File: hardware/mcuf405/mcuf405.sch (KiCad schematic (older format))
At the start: 35 parts, among them J4 STM32WORLD_BASE, U1 STM32F405RGTx, U2 XC6206P332MR, Y1 16 MHz

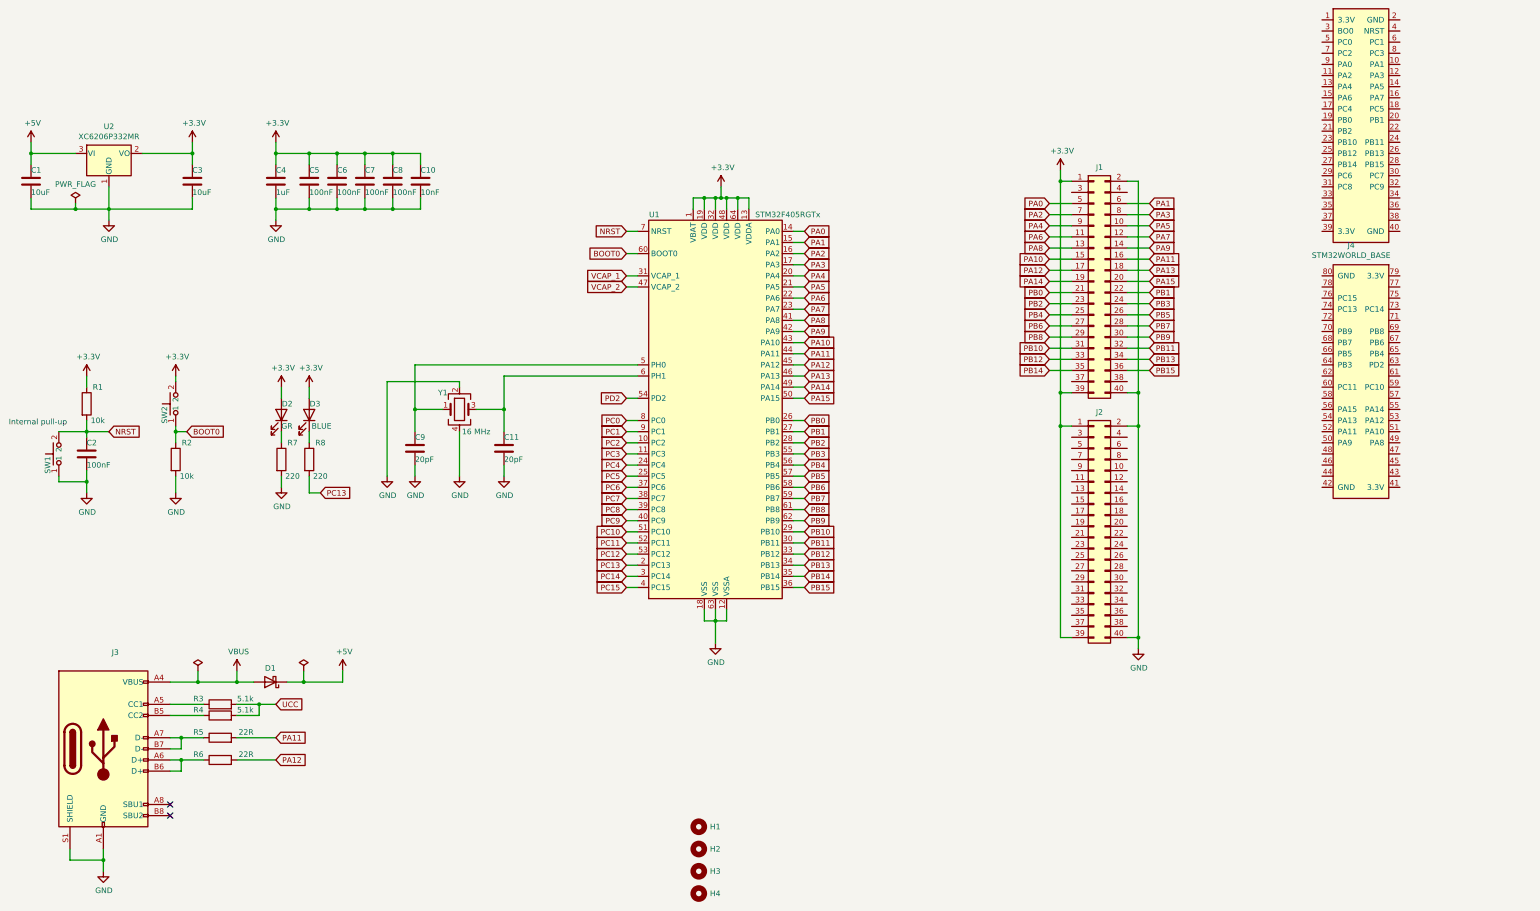
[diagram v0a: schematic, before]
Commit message: Hmmmm
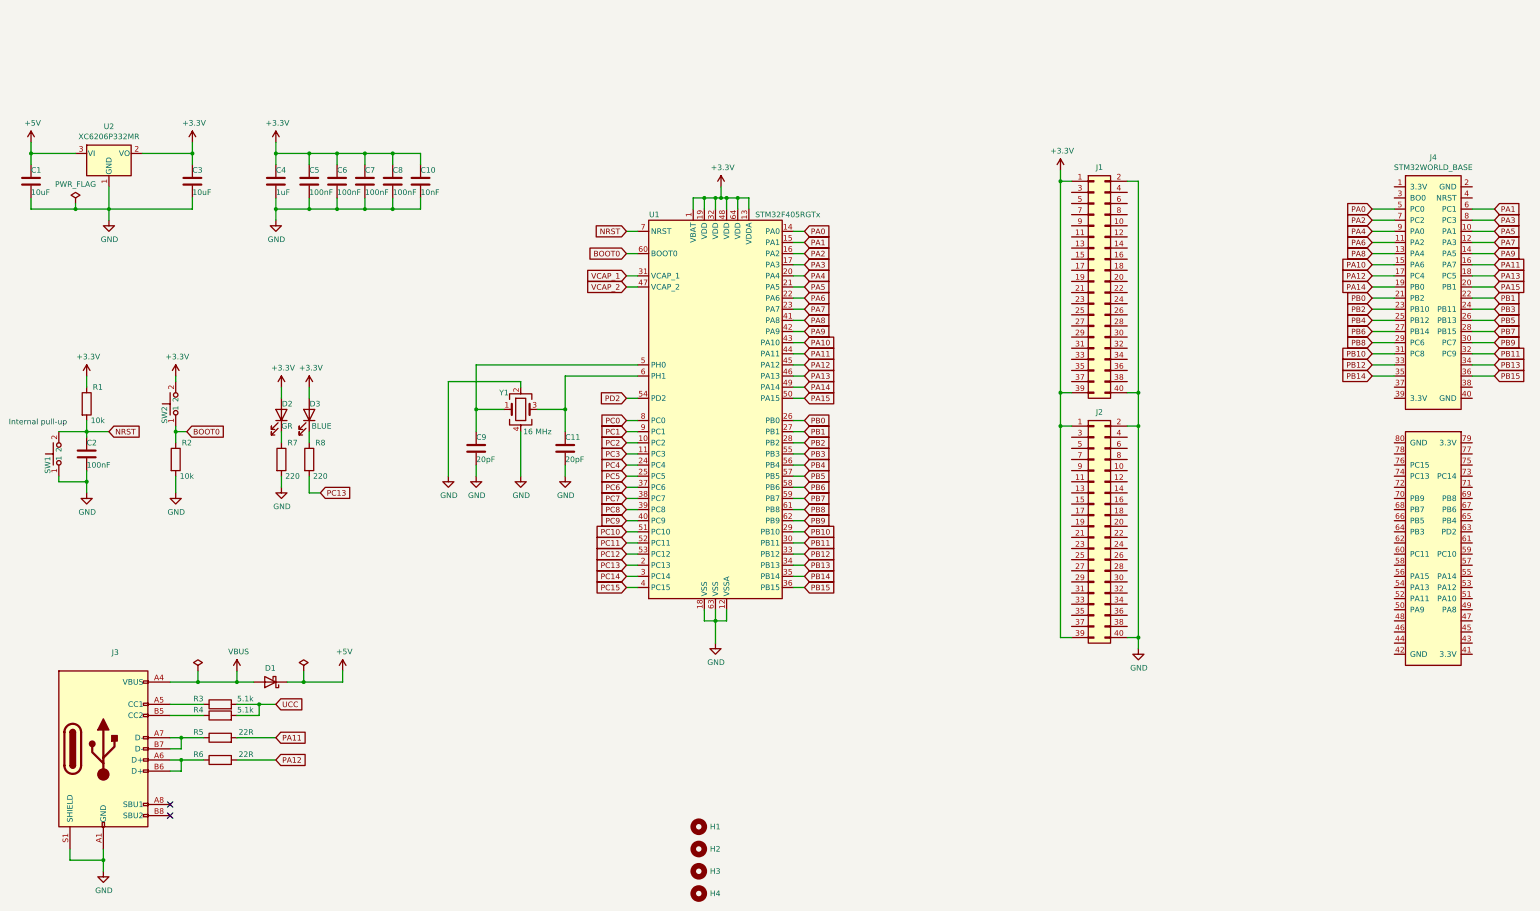
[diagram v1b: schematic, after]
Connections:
- net PA0: now also J4.5 (PC0); no longer J1.5 (Pin_5)
- net PA1: now also J4.6 (PC1); no longer J1.6 (Pin_6)
- net PA10: now also J4.15 (PA6); no longer J1.15 (Pin_15)
- net PA11: now also J4.16 (PA7); no longer J1.16 (Pin_16)
- net PA12: now also J4.17 (PC4); no longer J1.17 (Pin_17)
- net PA13: now also J4.18 (PC5); no longer J1.18 (Pin_18)
- net PA14: now also J4.19 (PB0); no longer J1.19 (Pin_19)
- net PA15: now also J4.20 (PB1); no longer J1.20 (Pin_20)
- net PA2: now also J4.7 (PC2); no longer J1.7 (Pin_7)
- net PA3: now also J4.8 (PC3); no longer J1.8 (Pin_8)
- net PA4: now also J4.9 (PA0); no longer J1.9 (Pin_9)
- net PA5: now also J4.10 (PA1); no longer J1.10 (Pin_10)
- net PA6: now also J4.11 (PA2); no longer J1.11 (Pin_11)
- net PA7: now also J4.12 (PA3); no longer J1.12 (Pin_12)
- net PA8: now also J4.13 (PA4); no longer J1.13 (Pin_13)
- net PA9: now also J4.14 (PA5); no longer J1.14 (Pin_14)
- net PB0: now also J4.21 (PB2); no longer J1.21 (Pin_21)
- net PB1: now also J4.22; no longer J1.22 (Pin_22)
- net PB10: now also J4.31 (PC8); no longer J1.31 (Pin_31)
- net PB11: now also J4.32 (PC9); no longer J1.32 (Pin_32)
- net PB12: now also J4.33; no longer J1.33 (Pin_33)
- net PB13: now also J4.34; no longer J1.34 (Pin_34)
- net PB14: now also J4.35; no longer J1.35 (Pin_35)
- net PB15: now also J4.36; no longer J1.36 (Pin_36)
- net PB2: now also J4.23 (PB10); no longer J1.23 (Pin_23)
- net PB3: now also J4.24 (PB11); no longer J1.24 (Pin_24)
- net PB4: now also J4.25 (PB12); no longer J1.25 (Pin_25)
- net PB5: now also J4.26 (PB13); no longer J1.26 (Pin_26)
- net PB6: now also J4.27 (PB14); no longer J1.27 (Pin_27)
- net PB7: now also J4.28 (PB15); no longer J1.28 (Pin_28)
- net PB8: now also J4.29 (PC6); no longer J1.29 (Pin_29)
- net PB9: now also J4.30 (PC7); no longer J1.30 (Pin_30)
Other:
- moved on the sheet: C11, C9, Y1

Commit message: Hmmmm
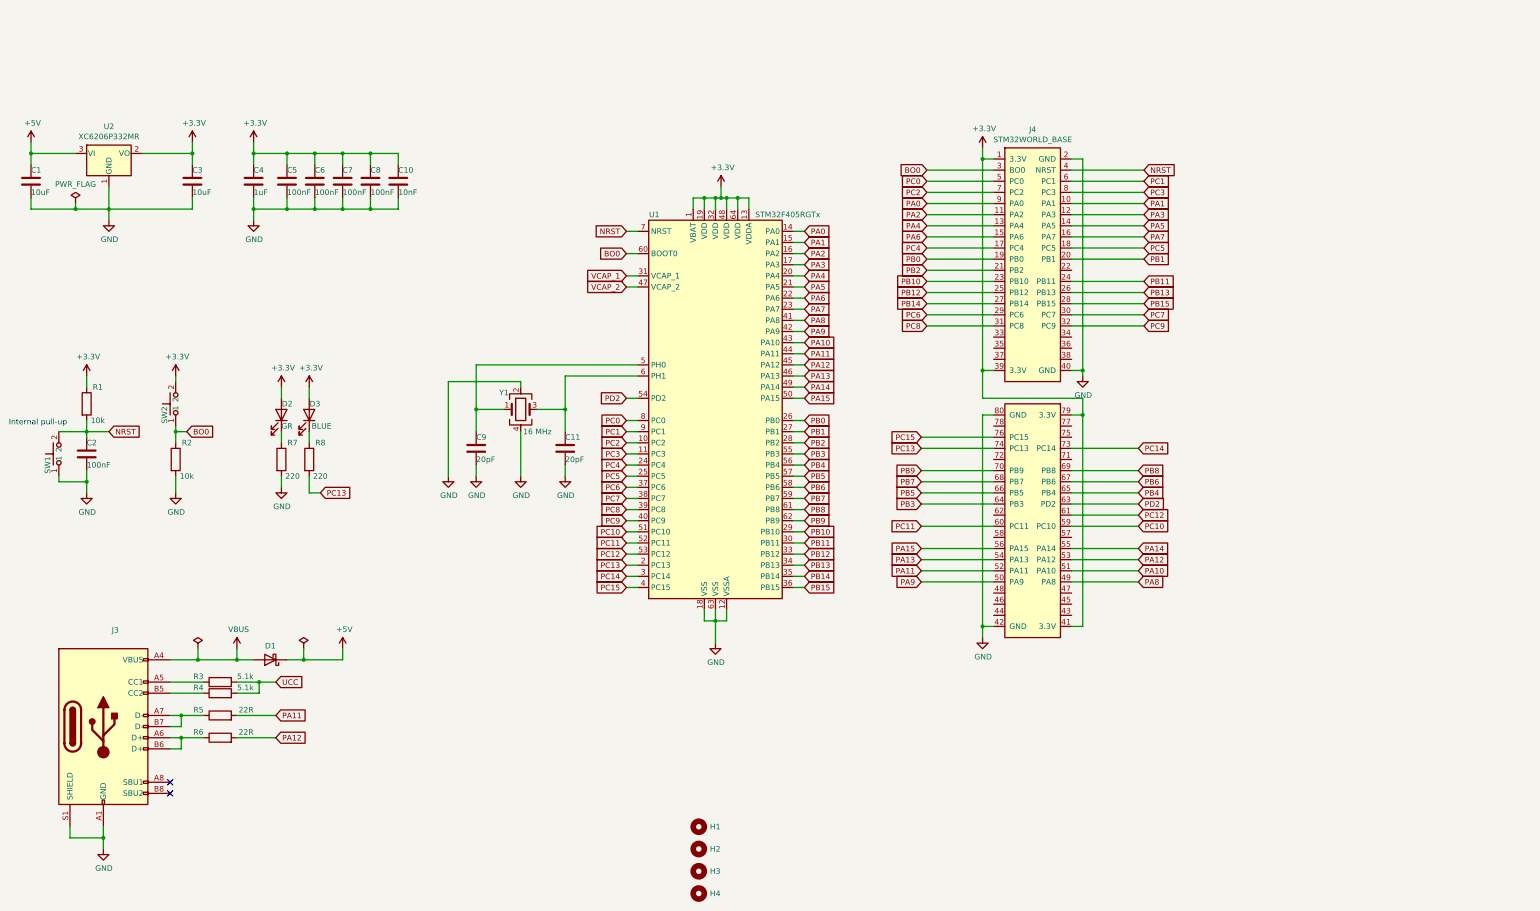
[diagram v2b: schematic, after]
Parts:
- removed J1, J2: ~, stm32world:PinSocket_2x20_P2.54mm_Vertical_Stackable, symbol Connector_Generic:Conn_02x20_Odd_Even
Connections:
- net BOOT0 is gone; now on net BO0: R2.1, SW2.1, U1.60 (BOOT0)
- net +3V3: now also J4.1 (3.3V), J4.39 (3.3V), J4.41 (3.3V), J4.79 (3.3V)
- net GND: now also J4.2 (GND), J4.40 (GND), J4.42 (GND), J4.80 (GND)
- net NRST: now also J4.4 (NRST)
- net PA0: now also J4.9 (PA0); no longer J4.5 (PC0)
- net PA1: now also J4.10 (PA1); no longer J4.6 (PC1)
- net PA10: now also J4.51 (PA10); no longer J4.15 (PA6)
- net PA11: now also J4.52 (PA11); no longer J4.16 (PA7)
- net PA12: now also J4.53 (PA12); no longer J4.17 (PC4)
- net PA13: now also J4.54 (PA13); no longer J4.18 (PC5)
- net PA14: now also J4.55 (PA14); no longer J4.19 (PB0)
- net PA15: now also J4.56 (PA15); no longer J4.20 (PB1)
- net PA2: now also J4.11 (PA2); no longer J4.7 (PC2)
- net PA3: now also J4.12 (PA3); no longer J4.8 (PC3)
- net PA4: now also J4.13 (PA4); no longer J4.9 (PA0)
- net PA5: now also J4.14 (PA5); no longer J4.10 (PA1)
- net PA6: now also J4.15 (PA6); no longer J4.11 (PA2)
- net PA7: now also J4.16 (PA7); no longer J4.12 (PA3)
- net PA8: now also J4.49 (PA8); no longer J4.13 (PA4)
- net PA9: now also J4.50 (PA9); no longer J4.14 (PA5)
- net PB0: now also J4.19 (PB0); no longer J4.21 (PB2)
- net PB1: now also J4.20 (PB1); no longer J4.22
- net PB10: now also J4.23 (PB10); no longer J4.31 (PC8)
- net PB11: now also J4.24 (PB11); no longer J4.32 (PC9)
- net PB12: now also J4.25 (PB12); no longer J4.33
- net PB13: now also J4.26 (PB13); no longer J4.34
- net PB14: now also J4.27 (PB14); no longer J4.35
- net PB15: now also J4.28 (PB15); no longer J4.36
- net PB2: now also J4.21 (PB2); no longer J4.23 (PB10)
- net PB3: now also J4.64 (PB3); no longer J4.24 (PB11)
- net PB4: now also J4.65 (PB4); no longer J4.25 (PB12)
- net PB5: now also J4.66 (PB5); no longer J4.26 (PB13)
- net PB6: now also J4.67 (PB6); no longer J4.27 (PB14)
- net PB7: now also J4.68 (PB7); no longer J4.28 (PB15)
- net PB8: now also J4.69 (PB8); no longer J4.29 (PC6)
- net PB9: now also J4.70 (PB9); no longer J4.30 (PC7)
- net PC0: now also J4.5 (PC0)
- net PC1: now also J4.6 (PC1)
- net PC10: now also J4.59 (PC10)
- net PC11: now also J4.60 (PC11)
- net PC12: now also J4.61
- net PC13: now also J4.74 (PC13)
- net PC14: now also J4.73 (PC14)
- net PC15: now also J4.76 (PC15)
- net PC2: now also J4.7 (PC2)
- net PC3: now also J4.8 (PC3)
- net PC4: now also J4.17 (PC4)
- net PC5: now also J4.18 (PC5)
- net PC6: now also J4.29 (PC6)
- net PC7: now also J4.30 (PC7)
- net PC8: now also J4.31 (PC8)
- net PC9: now also J4.32 (PC9)
- net PD2: now also J4.63 (PD2)
- net BO0: now reaches J4.3 (BO0)
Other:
- moved on the sheet: C10, C4, C5, C6, C7, C8, D1, J3, J4, R3, R4, R5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

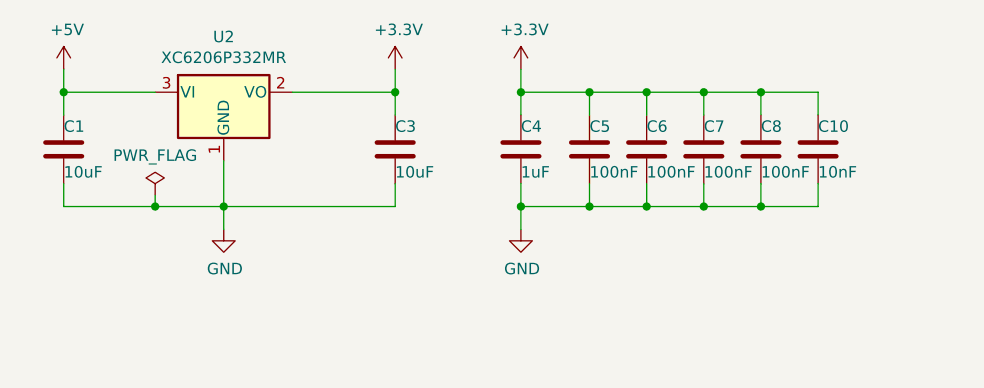
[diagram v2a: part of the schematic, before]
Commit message: Hmmmm
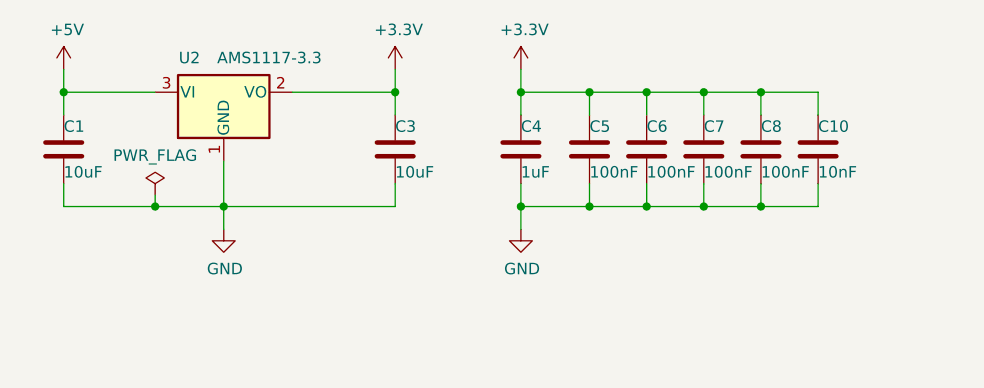
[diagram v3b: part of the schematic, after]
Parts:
- removed C5, C6, C7, C8: 100nF, Capacitor_SMD:C_0402_1005Metric, symbol Device:C
- removed U2: XC6206P332MR, Package_TO_SOT_SMD:SOT-23, symbol Regulator_Linear:XC6206PxxxMR
- added C5, C6, C7, C8: C_100NF_0603, Capacitor_SMD:C_0603_1608Metric, symbol stm32world:C_100NF_0603
- added U2: AMS1117-3.3, Package_TO_SOT_SMD:SOT-223-3_TabPin2, symbol stm32world:AMS1117-3.3
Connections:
- net +3V3: now also C5.1, C6.1, C7.1, C8.1, U2.2 (VO)
- net +5V: now also U2.3 (VI)
- net GND: now also C5.2, C6.2, C7.2, C8.2, U2.1 (GND)
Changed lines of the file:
@@
 	2750 5700 2900 5700
-$Comp
-L Device:C C?
-U 1 1 60D4188A
-P 3000 1200
-AR Path="/60D07374/60D4188A" Ref="C?"  Part="1"
-AR Path="/60D4188A" Ref="C5"  Part="1"
-F 0 "C5" H 3000 1300 50  0000 L CNN
-F 1 "100nF" H 3000 1100 50  0000 L CNN
-F 2 "Capacitor_SMD:C_0402_1005Metric" H 3038 1050 50  0001 C CNN
-F 3 "~" H 3000 1200 50  0001 C CNN
-F 4 "" H 3000 1200 50  0001 C CNN "LSCS"
-F 5 "C1525" H 3000 1200 50  0001 C CNN "LCSC"
-	1    3000 1200
-	1    0    0    -1
-$EndComp
 $Comp
 L power:GND #PWR?
@@
 	2700 950  2700 850
 Connection ~ 3000 950
-$Comp
-L Device:C C?
-U 1 1 60D418B8
-P 3250 1200
-AR Path="/60D07374/60D418B8" Ref="C?"  Part="1"
-AR Path="/60D418B8" Ref="C6"  Part="1"
-F 0 "C6" H 3250 1300 50  0000 L CNN
-F 1 "100nF" H 3250 1100 50  0000 L CNN
-F 2 "Capacitor_SMD:C_0402_1005Metric" H 3288 1050 50  0001 C CNN
-F 3 "~" H 3250 1200 50  0001 C CNN
-F 4 "" H 3250 1200 50  0001 C CNN "LSCS"
-F 5 "C1525" H 3250 1200 50  0001 C CNN "LCSC"
-	1    3250 1200
-	1    0    0    -1
-$EndComp
-$Comp
-L Device:C C?
-U 1 1 60D418C0
-P 3500 1200
-AR Path="/60D07374/60D418C0" Ref="C?"  Part="1"
-AR Path="/60D418C0" Ref="C7"  Part="1"
-F 0 "C7" H 3500 1300 50  0000 L CNN
-F 1 "100nF" H 3500 1100 50  0000 L CNN
-F 2 "Capacitor_SMD:C_0402_1005Metric" H 3538 1050 50  0001 C CNN
-F 3 "~" H 3500 1200 50  0001 C CNN
-F 4 "" H 3500 1200 50  0001 C CNN "LSCS"
-F 5 "C1525" H 3500 1200 50  0001 C CNN "LCSC"
-	1    3500 1200
-	1    0    0    -1
-$EndComp
-$Comp
-L Device:C C?
-U 1 1 60D418C8
-P 3750 1200
-AR Path="/60D07374/60D418C8" Ref="C?"  Part="1"
-AR Path="/60D418C8" Ref="C8"  Part="1"
-F 0 "C8" H 3750 1300 50  0000 L CNN
-F 1 "100nF" H 3750 1100 50  0000 L CNN
-F 2 "Capacitor_SMD:C_0402_1005Metric" H 3788 1050 50  0001 C CNN
-F 3 "~" H 3750 1200 50  0001 C CNN
-F 4 "" H 3750 1200 50  0001 C CNN "LSCS"
-F 5 "C1525" H 3750 1200 50  0001 C CNN "LCSC"
-	1    3750 1200
-	1    0    0    -1
-$EndComp
 Connection ~ 3000 1450
 Wire Wire Line
@@
 Wire Wire Line
 	2700 1450 3000 1450
-$Comp
-L Regulator_Linear:XC6206PxxxMR U?
-U 1 1 60D418E2
-P 1400 950
-AR Path="/60D07374/60D418E2" Ref="U?"  Part="1"
-AR Path="/60D418E2" Ref="U2"  Part="1"
-F 0 "U2" H 1400 1192 50  0000 C CNN
-F 1 "XC6206P332MR" H 1400 1101 50  0000 C CNN
-F 2 "Package_TO_SOT_SMD:SOT-23" H 1400 1175 50  0001 C CIN
-F 3 "https://www.torexsemi.com/file/xc6206/XC6206.pdf" H 1400 950 50  0001 C CNN
-F 4 "C5446" H 1400 950 50  0001 C CNN "LCSC"
-	1    1400 950
-	1    0    0    -1
-$EndComp
 $Comp
 L power:+3.3V #PWR?
@@
 	10150 5200 10050 5200
 Connection ~ 10150 3300
+$Comp
+L stm32world:AMS1117-3.3 U2
+U 1 1 60F141A5
+P 1400 950
+F 0 "U2" H 1250 1100 50  0000 C CNN
+F 1 "AMS1117-3.3" H 1600 1100 50  0000 C CNN
+F 2 "Package_TO_SOT_SMD:SOT-223-3_TabPin2" H 1400 1150 50  0001 C CNN
+F 3 "https://datasheet.lcsc.com/lcsc/1811142212_Advanced-Monolithic-Systems-AMS1117-3-3_C6186.pdf" H 1500 700 50  0001 C CNN
+F 4 "C6186" H 1550 700 50  0001 C CNN "LCSC"
+	1    1400 950
+	1    0    0    -1
+$EndComp
+$Comp
+L stm32world:C_100NF_0603 C5
+U 1 1 60EF1709
+P 3000 1200
+F 0 "C5" H 3000 1300 50  0000 L CNN
+F 1 "C_100NF_0603" H 3050 1050 50  0001 L CNN
+F 2 "Capacitor_SMD:C_0603_1608Metric" H 3700 950 50  0001 C CNN
+F 3 "~" H 3000 1200 50  0001 C CNN
+F 4 "100nF" H 3000 1100 50  0000 L CNN "Display"
+F 5 "C14663" H 3200 850 50  0001 C CNN "LCSC"
+	1    3000 1200
+	1    0    0    -1
+$EndComp
+$Comp
+L stm32world:C_100NF_0603 C6
+U 1 1 60EF316A
+P 3250 1200
+F 0 "C6" H 3250 1300 50  0000 L CNN
+F 1 "C_100NF_0603" H 3300 1050 50  0001 L CNN
+F 2 "Capacitor_SMD:C_0603_1608Metric" H 3950 950 50  0001 C CNN
+F 3 "~" H 3250 1200 50  0001 C CNN
+F 4 "100nF" H 3250 1100 50  0000 L CNN "Display"
+F 5 "C14663" H 3450 850 50  0001 C CNN "LCSC"
+	1    3250 1200
+	1    0    0    -1
+$EndComp
+$Comp
+L stm32world:C_100NF_0603 C7
+U 1 1 60EF3497
+P 3500 1200
+F 0 "C7" H 3500 1300 50  0000 L CNN
+F 1 "C_100NF_0603" H 3550 1050 50  0001 L CNN
+F 2 "Capacitor_SMD:C_0603_1608Metric" H 4200 950 50  0001 C CNN
+F 3 "~" H 3500 1200 50  0001 C CNN
+F 4 "100nF" H 3500 1100 50  0000 L CNN "Display"
+F 5 "C14663" H 3700 850 50  0001 C CNN "LCSC"
+	1    3500 1200
+	1    0    0    -1
+$EndComp
+$Comp
+L stm32world:C_100NF_0603 C8
+U 1 1 60EF3928
+P 3750 1200
+F 0 "C8" H 3750 1300 50  0000 L CNN
+F 1 "C_100NF_0603" H 3800 1050 50  0001 L CNN
+F 2 "Capacitor_SMD:C_0603_1608Metric" H 4450 950 50  0001 C CNN
+F 3 "~" H 3750 1200 50  0001 C CNN
+F 4 "100nF" H 3750 1100 50  0000 L CNN "Display"
+F 5 "C14663" H 3950 850 50  0001 C CNN "LCSC"
+	1    3750 1200
+	1    0    0    -1
+$EndComp
 $EndSCHEMATC
